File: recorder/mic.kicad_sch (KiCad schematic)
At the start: 3 parts, among them U1 IM73D122V01

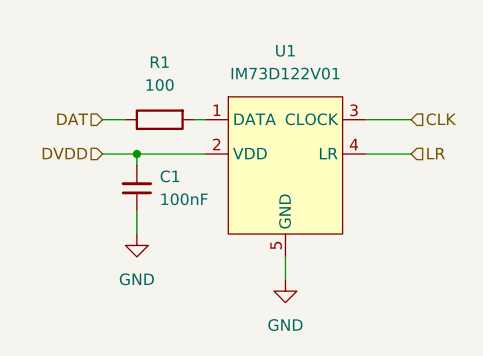
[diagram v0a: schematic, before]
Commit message: MPN and Package
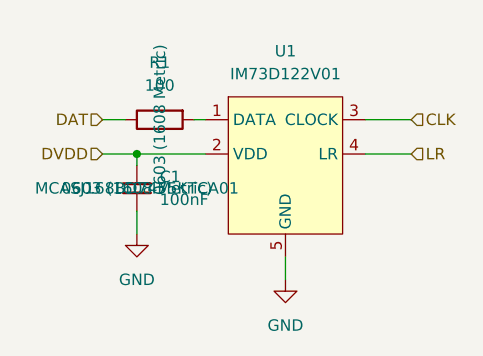
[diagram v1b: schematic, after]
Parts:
- C1: MPN (none) -> MCASJ168BD7475KTCA01; Package (none) -> 0603 (1608 Metric)
- R1: Package (none) -> 0603 (1608 Metric)
- U1: MPN (none) -> IM73D122V01XTMA1; Manufacturer (none) -> Infineon Technologies; Package (none) -> LGA-5
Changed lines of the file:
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@@
+			)
+		)
+		(property "Manufacturer" "Infineon Technologies"
+			(at 139.7 85.09 0)
+			(effects
+				(font
+					(size 1.27 1.27)
+				)
+				(hide yes)
+			)
+		)
+		(property "MPN" "IM73D122V01XTMA1"
+			(at 139.7 85.09 0)
+			(effects
+				(font
+					(size 1.27 1.27)
+				)
+				(hide yes)
+			)
+		)
+		(property "Package" "LGA-5"
+			(at 139.7 85.09 0)
+			(effects
+				(font
+					(size 1.27 1.27)
+				)
+				(hide yes)
 			)
 		)
@@
 			)
 		)
+		(property "Package" "0603 (1608 Metric)"
+			(at 125.73 80.01 0)
+			(effects
+				(font
+					(size 1.27 1.27)
+				)
+			)
+		)
 		(pin "2"
 		)
@@
 			)
 		)
+		(property "MPN" "MCASJ168BD7475KTCA01"
+			(at 123.19 87.63 0)
+			(effects
+				(font
+					(size 1.27 1.27)
+				)
+			)
+		)
+		(property "Package" "0603 (1608 Metric)"
+			(at 123.19 87.63 0)
+			(effects
+				(font
+					(size 1.27 1.27)
+				)
+			)
+		)
